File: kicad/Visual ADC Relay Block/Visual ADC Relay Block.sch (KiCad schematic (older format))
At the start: 34 parts, among them J1 Out, J2 In, K1 DIPxx-1Cxx-51x, Q1 P-NMOS, U1 74HCT595, U2 74HC245

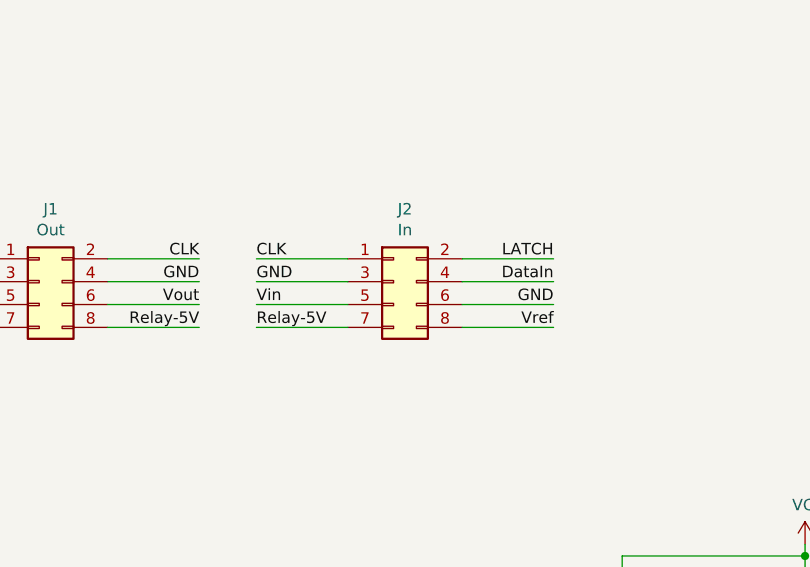
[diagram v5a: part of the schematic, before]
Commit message: pass DRC yay!
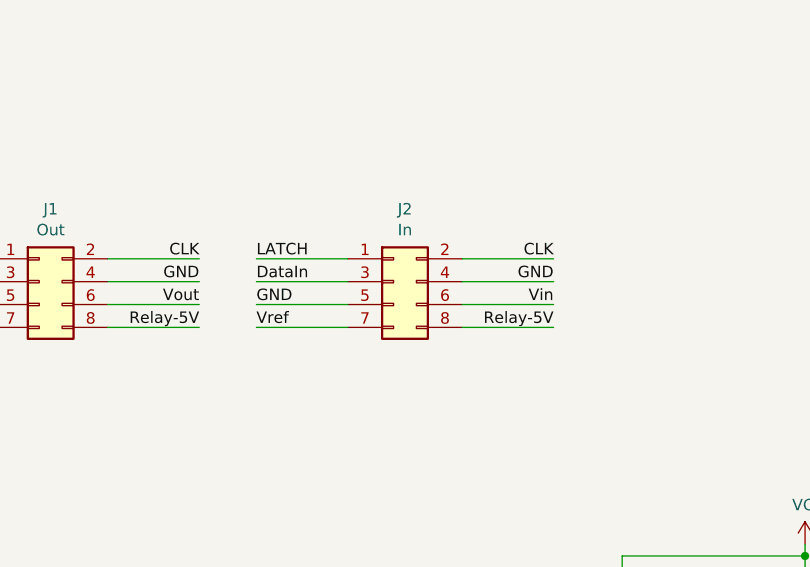
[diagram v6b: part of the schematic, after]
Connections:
- net CLK: now also J2.2 (Pin_2); no longer J2.1 (Pin_1)
- net DataIn: now also J2.3 (Pin_3); no longer J2.4 (Pin_4)
- net GND: now also J2.4 (Pin_4), J2.5 (Pin_5); no longer J2.3 (Pin_3), J2.6 (Pin_6)
- net LATCH: now also J2.1 (Pin_1); no longer J2.2 (Pin_2)
- net VCC: now also J2.8 (Pin_8); no longer J2.7 (Pin_7)
- net Vin: now also J2.6 (Pin_6); no longer J2.5 (Pin_5)
- net Vref: now also J2.7 (Pin_7); no longer J2.8 (Pin_8)
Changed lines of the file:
@@
 Text Label 14900 8400 3    50   ~ 0
 LED6
-$Comp
-L Connector_Generic:Conn_02x04_Odd_Even J2
-U 1 1 603C4B3A
-P 8350 6850
-F 0 "J2" H 8400 7167 50  0000 C CNN
-F 1 "In" H 8400 7076 50  0000 C CNN
-F 2 "Connector_PinHeader_2.54mm:PinHeader_2x04_P2.54mm_Vertical" H 8350 6850 50  0001 C CNN
-F 3 "~" H 8350 6850 50  0001 C CNN
-	1    8350 6850
-	1    0    0    -1
-$EndComp
 Wire Wire Line
 	6600 6850 6200 6850
@@
 Text Label 15200 9100 3    50   ~ 0
 CL4
-Wire Wire Line
-	8150 7050 7750 7050
-Wire Wire Line
-	7750 6850 8150 6850
-Wire Wire Line
-	9050 7050 8650 7050
-Wire Wire Line
-	7750 6950 8150 6950
-Text Label 9050 7050 2    50   ~ 0
-Vref
-Text Label 7750 7050 0    50   ~ 0
-Relay-5V
-Text Label 9050 6950 2    50   ~ 0
-GND
-Wire Wire Line
-	8650 6950 9050 6950
-Text Label 9050 6750 2    50   ~ 0
-LATCH
-Wire Wire Line
-	8650 6750 9050 6750
-Text Label 7750 6750 0    50   ~ 0
-CLK
-Wire Wire Line
-	8150 6750 7750 6750
-Text Label 9050 6850 2    50   ~ 0
-DataIn
-Wire Wire Line
-	8650 6850 9050 6850
 Text Label 6200 6950 0    50   ~ 0
-GND
-Text Label 7750 6850 0    50   ~ 0
 GND
 Text Label 7500 6950 2    50   ~ 0
 Vout
+$Comp
+L Connector_Generic:Conn_02x04_Odd_Even J2
+U 1 1 603C4B3A
+P 8350 6850
+F 0 "J2" H 8400 7167 50  0000 C CNN
+F 1 "In" H 8400 7076 50  0000 C CNN
+F 2 "Connector_PinHeader_2.54mm:PinHeader_2x04_P2.54mm_Vertical" H 8350 6850 50  0001 C CNN
+F 3 "~" H 8350 6850 50  0001 C CNN
+	1    8350 6850
+	1    0    0    -1
+$EndComp
+Wire Wire Line
+	8150 6850 7750 6850
+Text Label 7750 6850 0    50   ~ 0
+DataIn
+Wire Wire Line
+	8150 6750 7750 6750
+Text Label 7750 6750 0    50   ~ 0
+LATCH
+Wire Wire Line
+	8150 6950 7750 6950
 Text Label 7750 6950 0    50   ~ 0
+GND
+Text Label 7750 7050 0    50   ~ 0
+Vref
+Wire Wire Line
+	7750 7050 8150 7050
+Text Label 9050 6950 2    50   ~ 0
 Vin
+Text Label 9050 6850 2    50   ~ 0
+GND
+Wire Wire Line
+	8650 6750 9050 6750
+Text Label 9050 6750 2    50   ~ 0
+CLK
+Text Label 9050 7050 2    50   ~ 0
+Relay-5V
+Wire Wire Line
+	9050 6950 8650 6950
+Wire Wire Line
+	9050 6850 8650 6850
+Wire Wire Line
+	8650 7050 9050 7050
 $EndSCHEMATC
